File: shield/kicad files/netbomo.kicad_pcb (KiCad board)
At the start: 2 copper layers, 53 parts, among them CON1 BARREL_JACK, J1 JACK_STEREO, P1 WIND1, P2 WIND2, P3 VANE, P5 WIND2/RFM, U1 LM358, U2 LM358, U3 RFM12

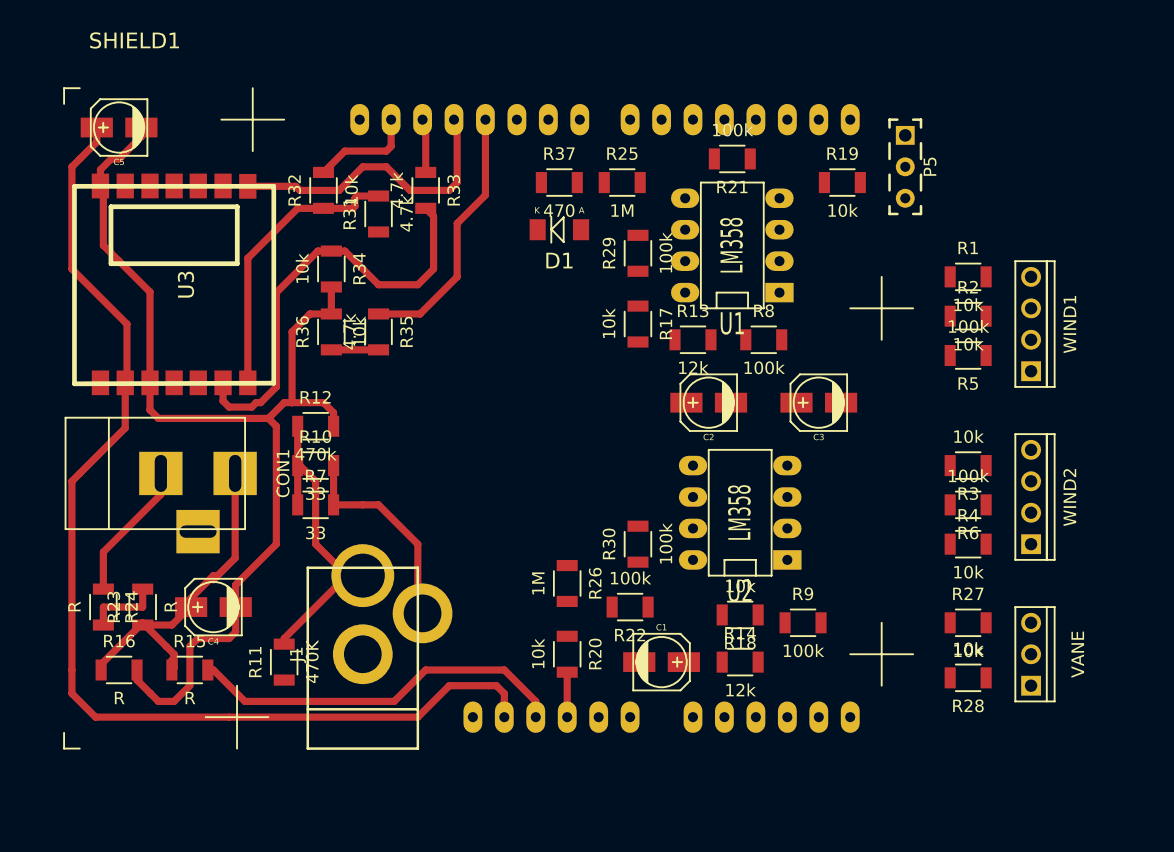
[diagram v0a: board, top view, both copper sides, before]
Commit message: update kicad files
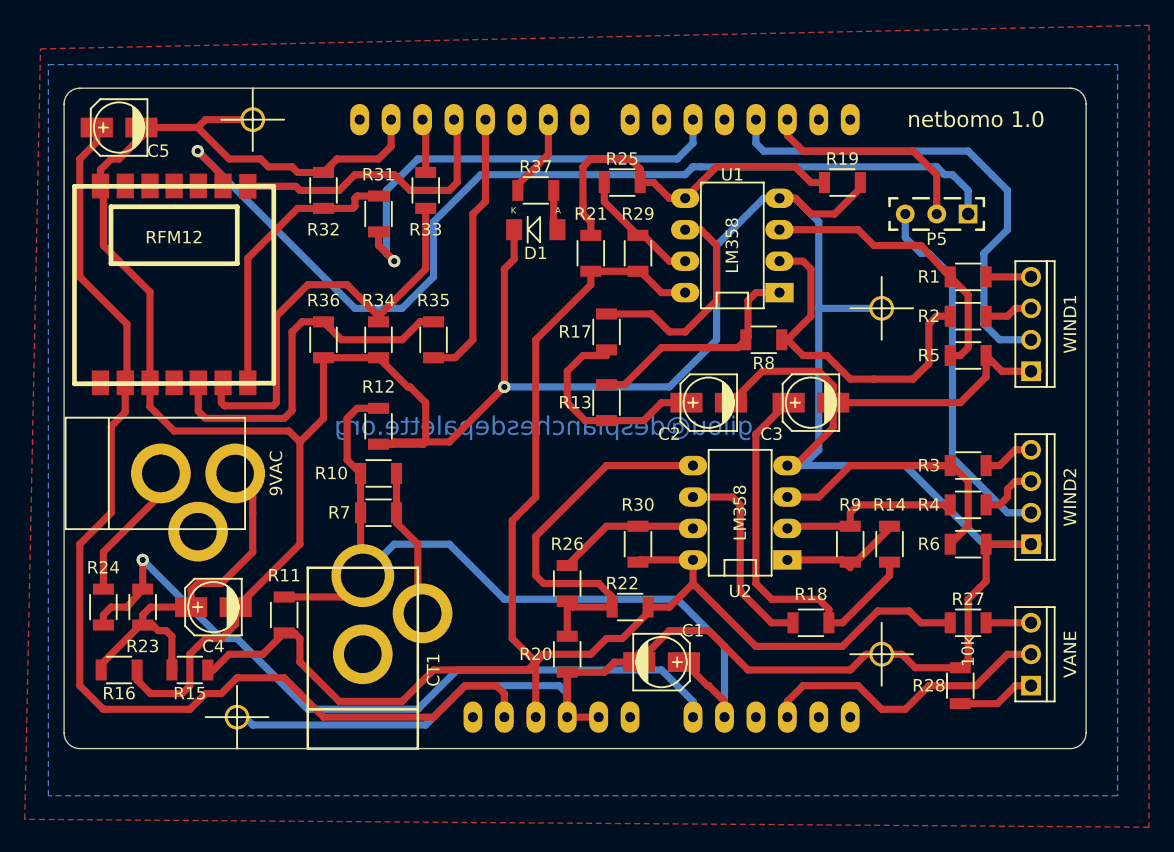
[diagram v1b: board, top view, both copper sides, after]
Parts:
- removed CON1: BARREL_JACK, Connect:BARREL_JACK
- removed J1: JACK_STEREO, diy_connectors:JACK_2.1_DC
- removed SHIELD1: ARDUINO_SHIELD, Arduino:ARDUINO_SHIELD_2
- removed U3: RFM12, rfm12:RFM12
- added 9VAC: BARREL_JACK, Connect:BARREL_JACK, F.Cu at (94.0, 62.9)
- added CT1: JACK_STEREO, diy_connectors:JACK_2.1_DC, F.Cu at (110.5, 77.5)
- added RFM12: RFM12, rfm12:RFM12, F.Cu at (95.2, 47.6)
- added netbomo 1.0: ARDUINO_SHIELD, Arduino:ARDUINO_SHIELD_2, F.Cu at (86.4, 85.1)
- moved R14 15.4 mm to (153.0, 68.6), turned to 90 degrees
- moved R21 13.7 mm to (128.9, 45.1), turned to 90 degrees
- moved R13 8.64 mm to (130.2, 57.1), turned to 90 degrees
- moved R9 7.41 mm to (149.9, 68.6), turned to 90 degrees
- moved R34 6.87 mm to (111.8, 52.1)
- moved R18 5.75 mm to (146.7, 74.9), turned to 0 degrees
- moved R10 5.12 mm to (111.8, 62.9)
- moved R7 5.12 mm to (111.8, 66.0)
- moved R12 5.08 mm to (111.8, 59.1), turned to 270 degrees
- moved P5 4.58 mm to (156.8, 41.9), turned to 180 degrees
- moved R35 4.49 mm to (116.2, 52.1), turned to 90 degrees
- moved R11 3.81 mm to (104.1, 74.3)
- moved R4 3.17 mm to (159.4, 65.4)
- moved R6 3.17 mm to (159.4, 68.6)
- moved R17 2.62 mm to (130.2, 51.4)
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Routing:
- net GND: track 99.6 -> 372.0 mm, vias 0 -> 1
- net +5V: track 30.9 -> 128.0 mm
- net Net-(P5-Pad1): track 0.00 -> 81.2 mm, vias 0 -> 1
- net /ADC0: track 6.08 -> 60.4 mm, vias 0 -> 1
- net /ADC1: track 27.2 -> 68.4 mm
- net /DIG3: track 0.00 -> 39.7 mm
- net /DIG5: track 0.00 -> 37.1 mm, vias 0 -> 1
- net Net-(R20-Pad1): track 0.00 -> 32.6 mm
- net Net-(C3-Pad1): track 0.00 -> 31.2 mm
- net /ANEMO2: track 0.00 -> 29.8 mm
- net Net-(R19-Pad1): track 0.00 -> 29.1 mm
- net Net-(R2-Pad1): track 0.00 -> 28.2 mm
- net Net-(R35-Pad2): track 3.81 -> 29.7 mm
- net /ADC3: track 0.00 -> 24.1 mm
- net Net-(R1-Pad1): track 0.00 -> 23.5 mm
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- added copper zone on B.Cu, net GND
- added copper zone on F.Cu, net GND
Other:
- board outline added: 82.6 x 53.3 mm
- board text added: "gilou@desplanchesdepalette.org"
